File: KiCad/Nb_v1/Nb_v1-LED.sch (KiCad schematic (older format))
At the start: 161 parts, among them K2 LED_ENABLE, Q1 2N5401, Q10 2N5401, Q11 2N5401, Q12 2N5401, Q13 2N5401, Q14 2N5401, Q15 2N5401, Q16 2N5401, Q2 2N5401, Q3 2N5401, Q4 2N5401, Q5 2N5401, Q6 2N5401, Q7 2N5401, Q8 2N5401, Q9 2N5401

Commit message: Nb_v1 Nachbau Schematic
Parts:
- removed K2: LED_ENABLE, pin_strip_3, symbol CONN_3
- removed Q1, Q10, Q11, Q12, Q13, Q14, Q15, Q16, Q2, Q3, Q4, Q5, Q6, Q7, Q8, Q9: 2N5401, to92_2N5401, symbol PNP
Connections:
- net labels added: R09, R10
- net labels removed: COL12, COL13, COL14, COL15, COL16, VCC
- wire segments 382 -> 402
- no-connect marks 1 -> 0
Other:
- moved on the sheet: D100, D101, D102, D103, D104, D105, D106, D107, D108, D109, D110, D111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

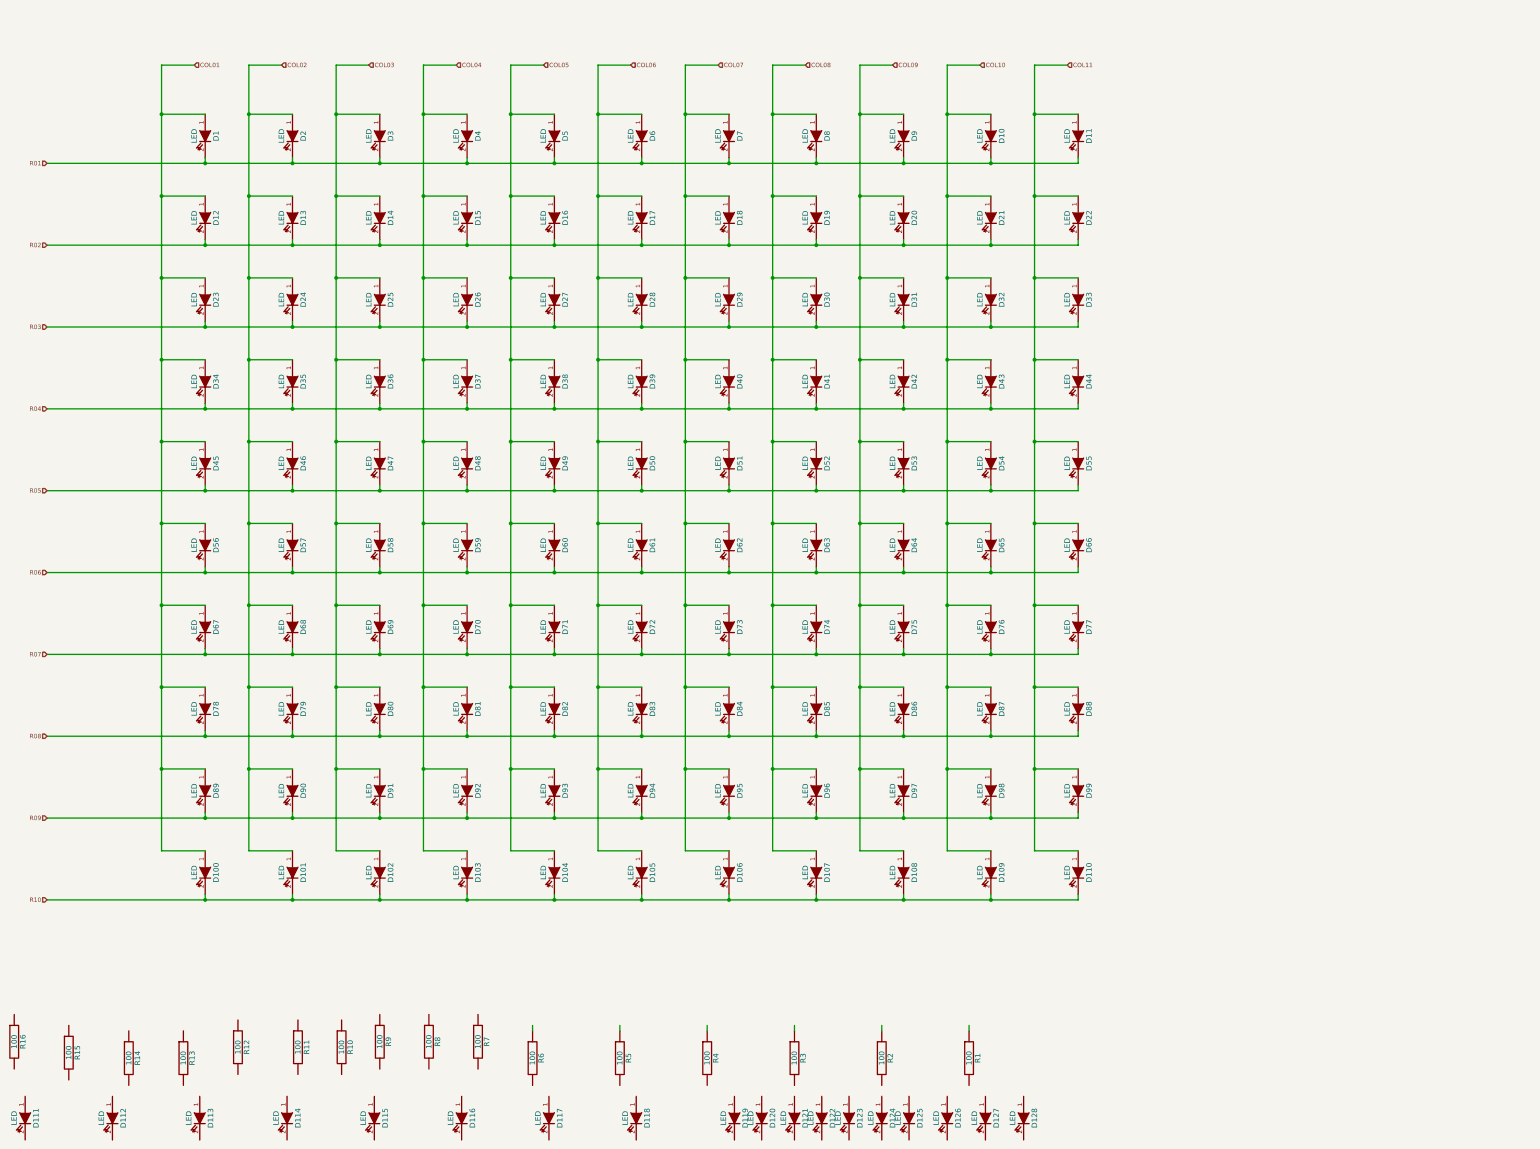
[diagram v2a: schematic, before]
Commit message: NachBau Schematic update
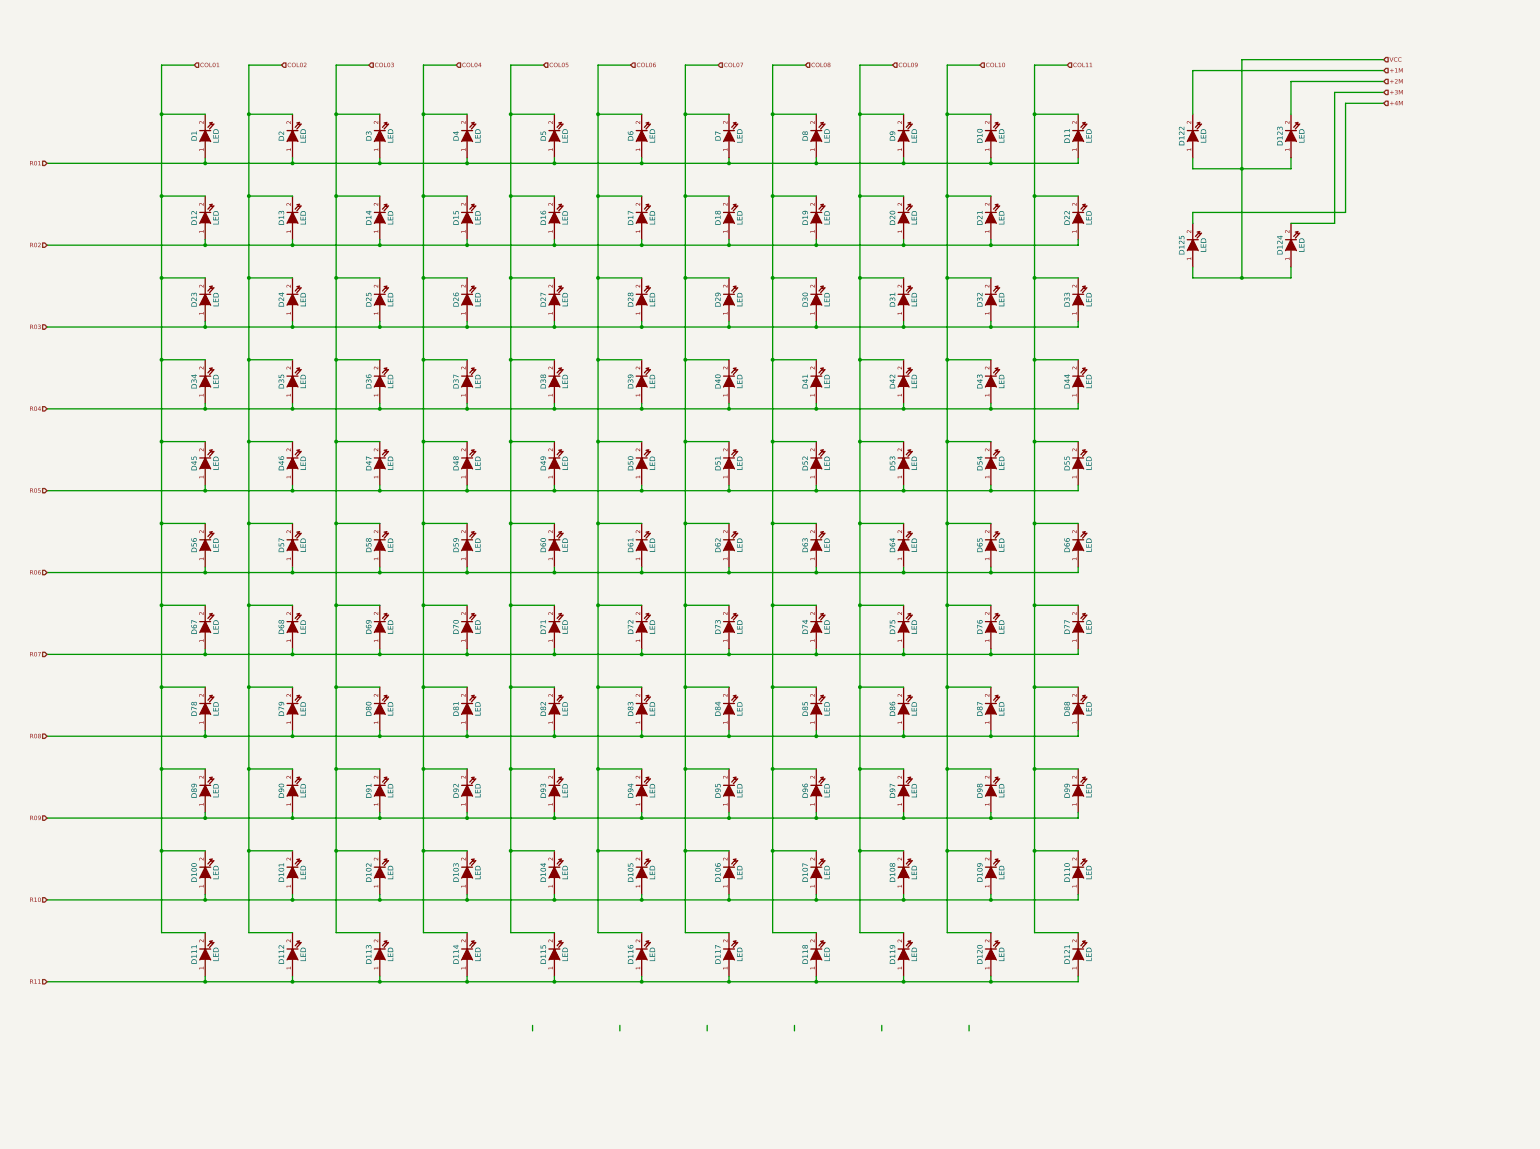
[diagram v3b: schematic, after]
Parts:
- removed D126, D127, D128: LED, led_5mm_clear, symbol LED
- removed R1, R10, R11, R12, R13, R14, R15, R16, R2, R3, R4, R5, R6, R7, R8, R9: 100, RC03, symbol R
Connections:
- net labels added: +1M, +2M, +3M, +4M, R11, VCC
- wire segments 402 -> 300
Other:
- moved on the sheet: D111, D112, D113, D114, D115, D116, D117, D118, D119, D120, D121
